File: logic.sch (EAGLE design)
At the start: 7 parts, among them CON1 PINHEAD_1X10-2, CON2 PINHEAD_1X10-2, CON3 PINHEAD_1X02-2, CON4 PINHEAD_1X02-2, CON5 PINHEAD_1X02-2, CON7 PINHEAD_1X07-2

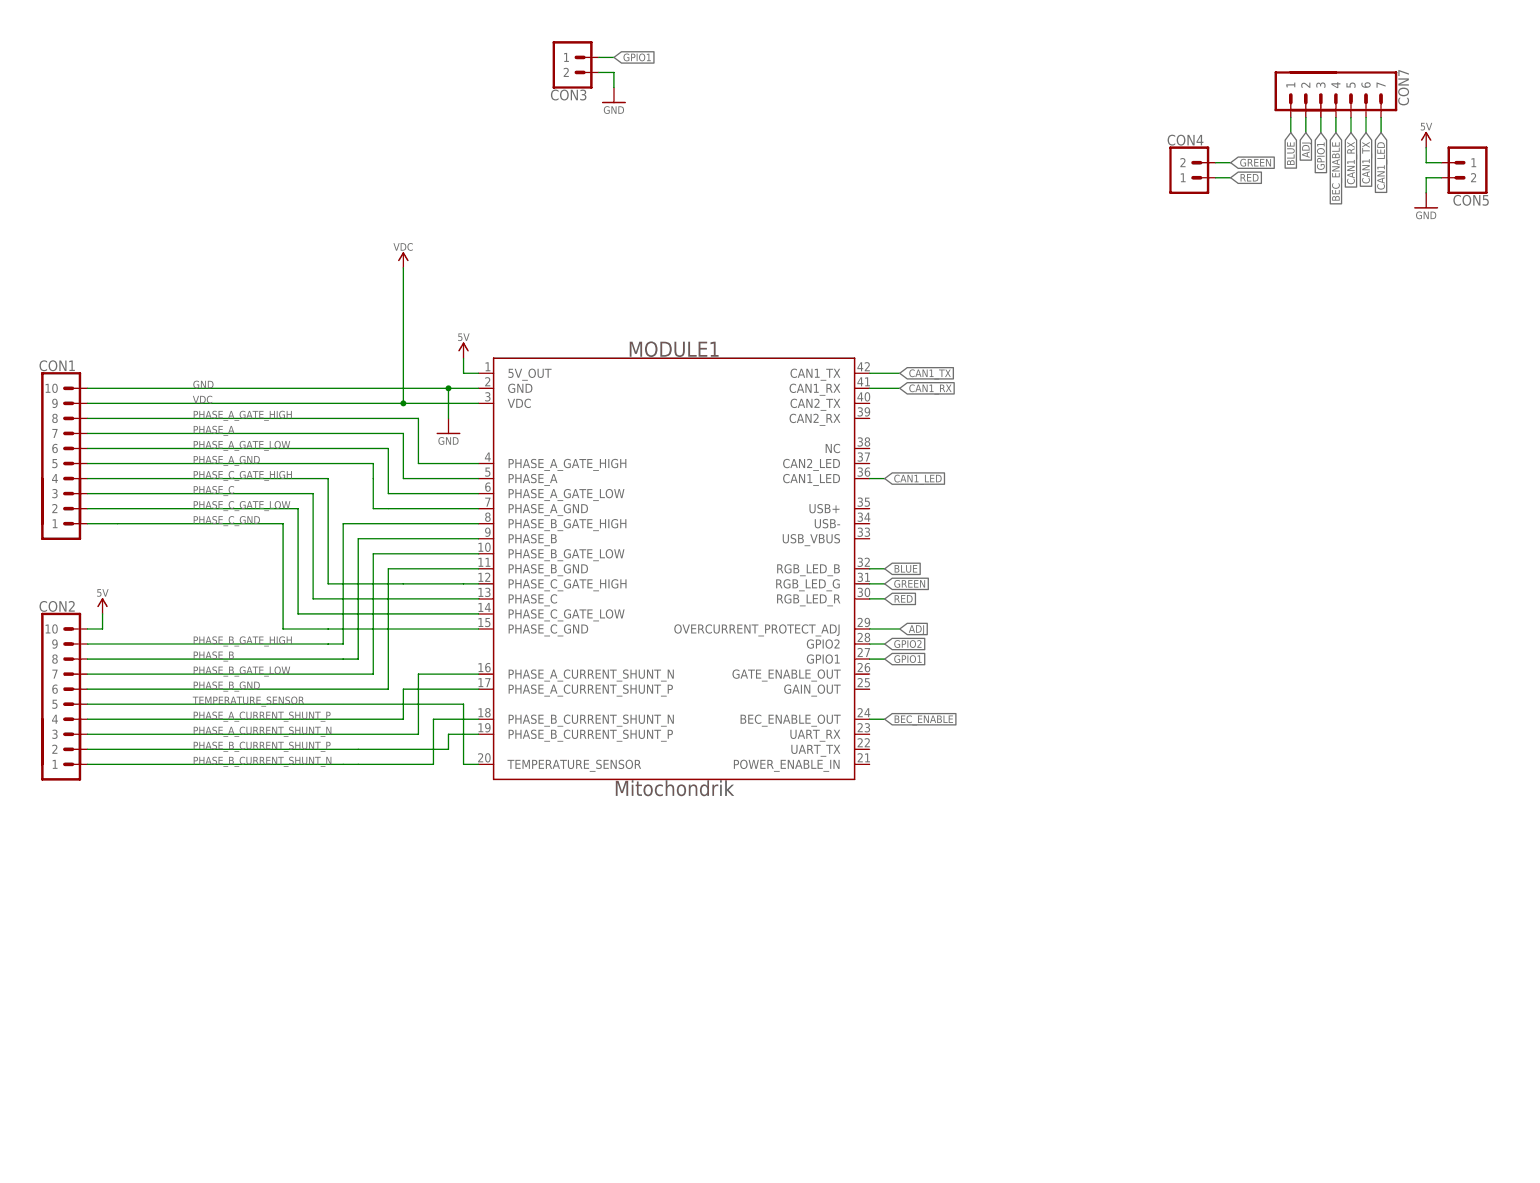
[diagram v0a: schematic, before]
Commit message: let there be a giant hole in the middle of the PCB
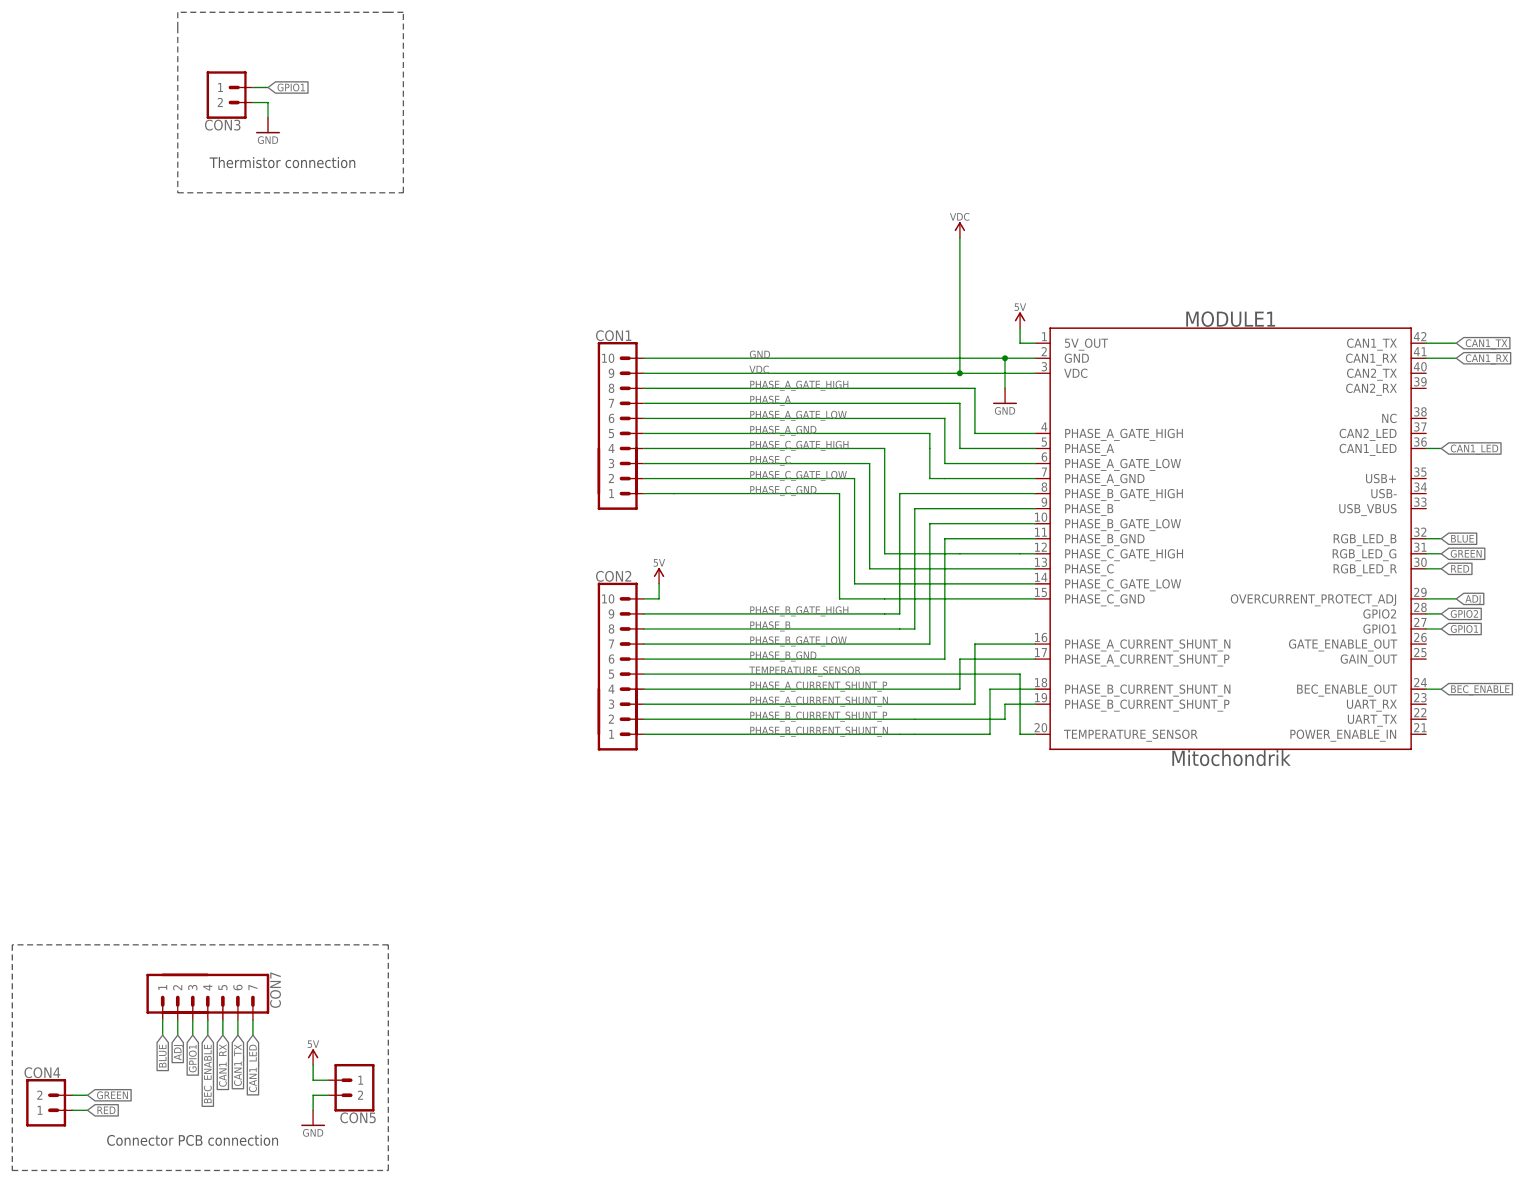
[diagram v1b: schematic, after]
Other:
- note added: "Connector PCB connection"
- note added: "Thermistor connection"
- moved on the sheet: CON1, CON2, CON3, CON4, CON5, CON7, MODULE1
